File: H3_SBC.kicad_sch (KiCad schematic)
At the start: 7 parts, among them U1 H3, U8 XOS32024000LT00351005, X1 X201232768KLD2SI

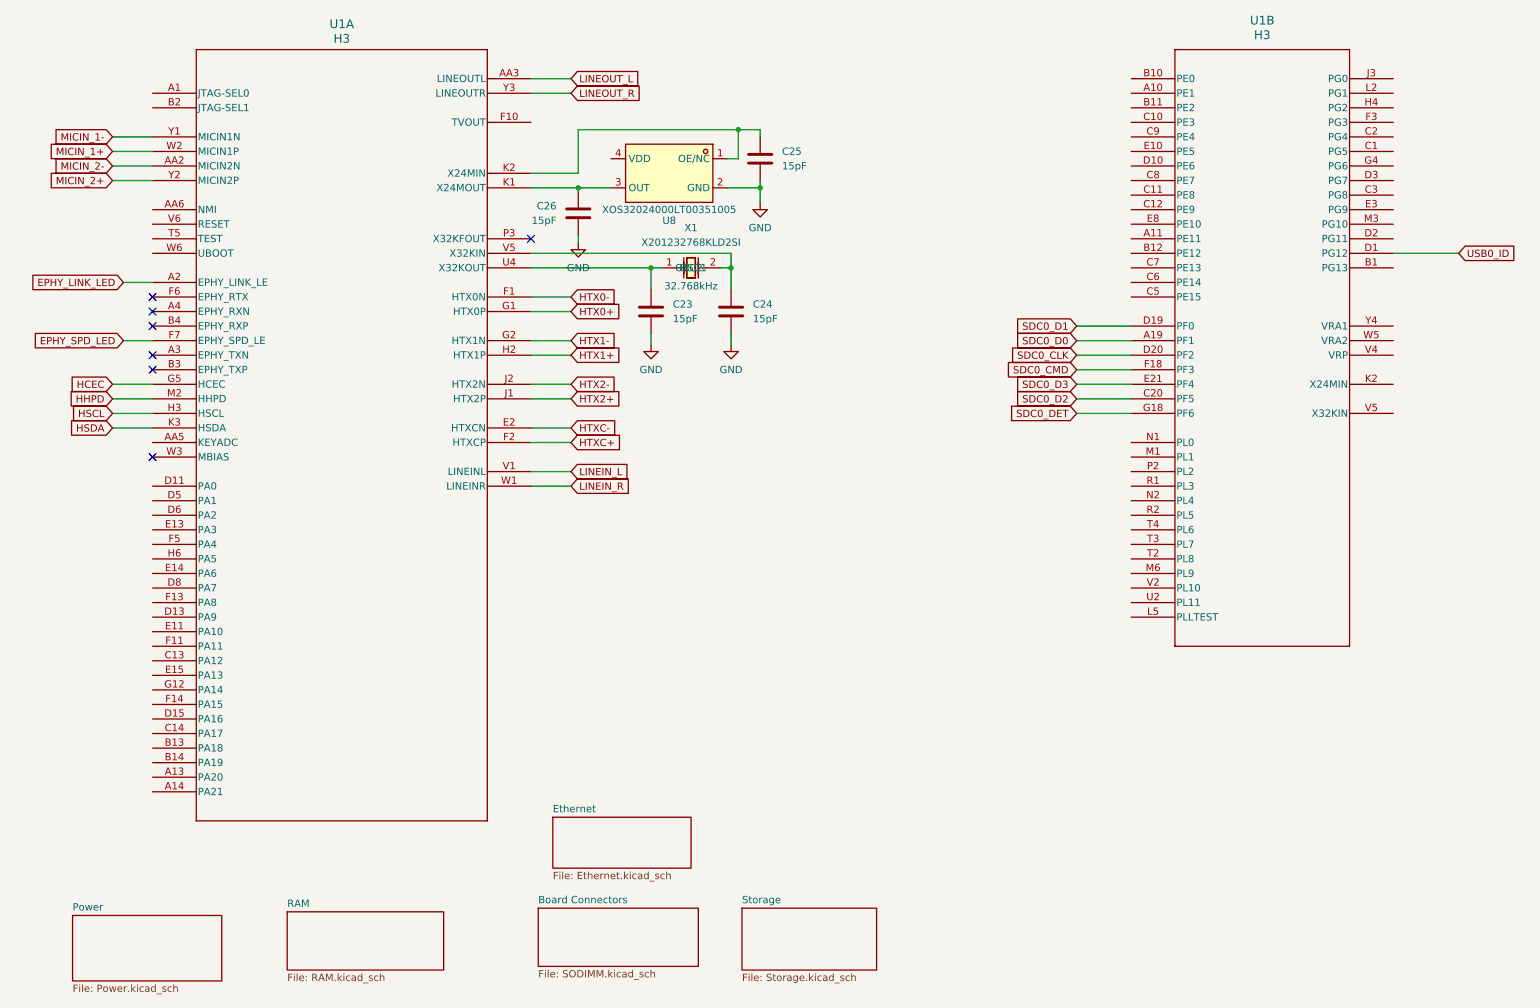
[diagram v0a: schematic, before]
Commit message: changed some ethernet stuff
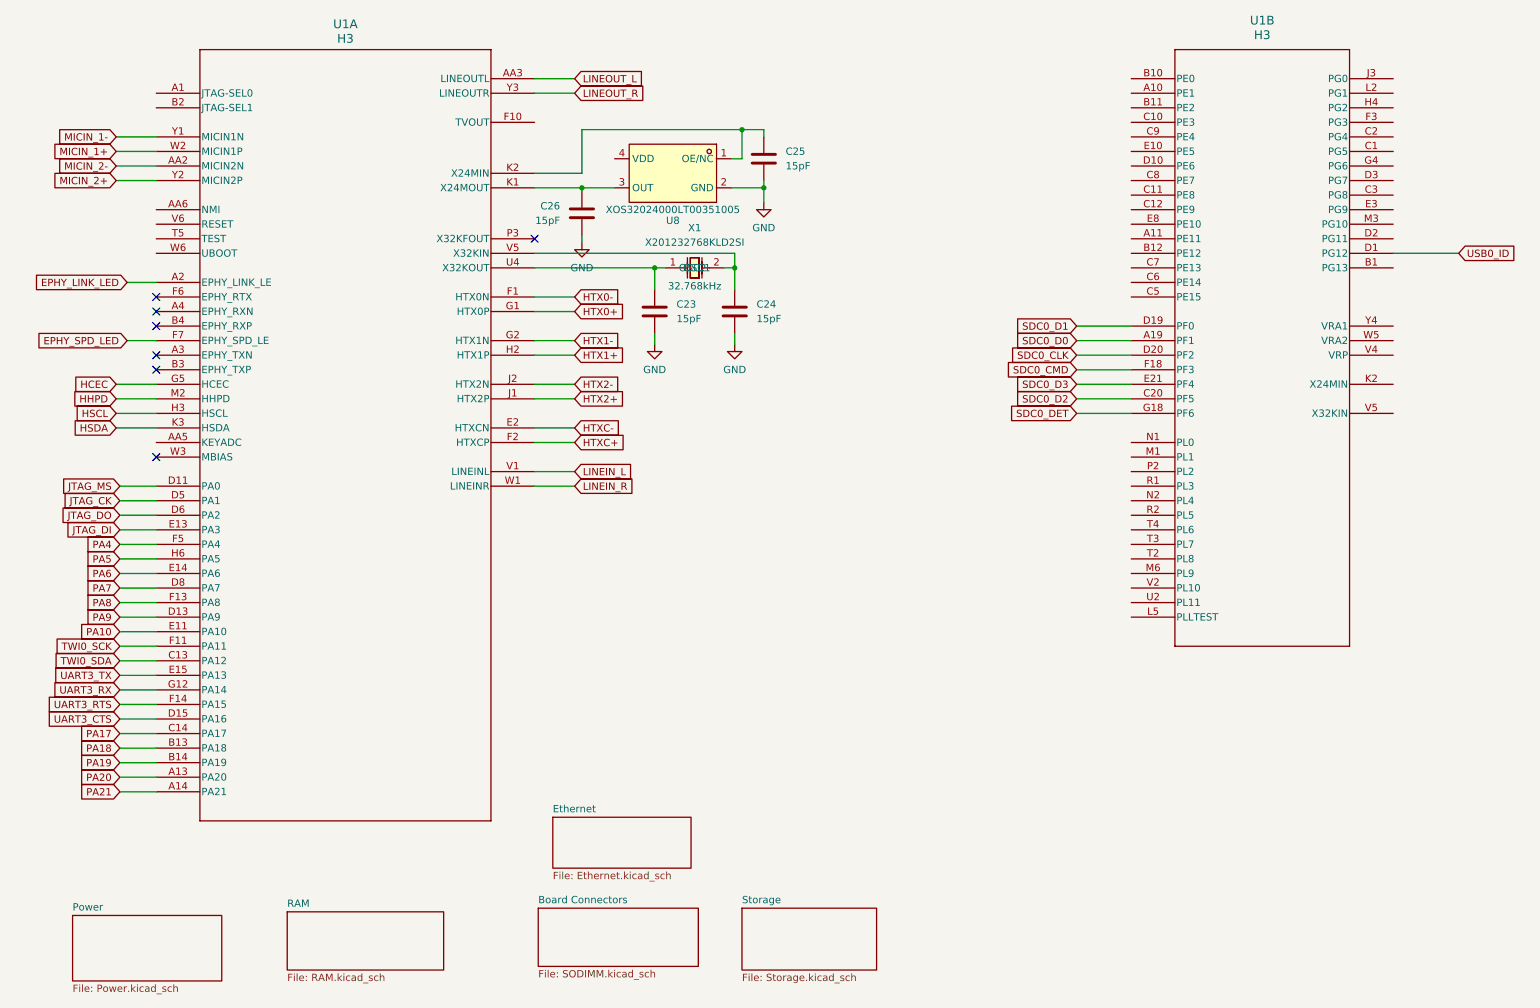
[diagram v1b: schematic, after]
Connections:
- net PA20: now reaches U1.A13 (PA20)
- net PA21: now reaches U1.A14 (PA21)
- net PA18: now reaches U1.B13 (PA18)
- net PA19: now reaches U1.B14 (PA19)
- net TWI0_SDA: now reaches U1.C13 (PA12)
- net PA17: now reaches U1.C14 (PA17)
- net JTAG_MS: now reaches U1.D11 (PA0)
- net PA9: now reaches U1.D13 (PA9)
- net UART3_CTS: now reaches U1.D15 (PA16)
- net JTAG_CK: now reaches U1.D5 (PA1)
- net JTAG_DO: now reaches U1.D6 (PA2)
- net PA7: now reaches U1.D8 (PA7)
- net PA10: now reaches U1.E11 (PA10)
- net JTAG_DI: now reaches U1.E13 (PA3)
- net PA6: now reaches U1.E14 (PA6)
- net UART3_TX: now reaches U1.E15 (PA13)
- net TWI0_SCK: now reaches U1.F11 (PA11)
- net PA8: now reaches U1.F13 (PA8)
- net UART3_RTS: now reaches U1.F14 (PA15)
- net PA4: now reaches U1.F5 (PA4)
- net UART3_RX: now reaches U1.G12 (PA14)
- net PA5: now reaches U1.H6 (PA5)
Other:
- moved on the sheet: C23, C24, C25, C26, U1A, U8, X1
